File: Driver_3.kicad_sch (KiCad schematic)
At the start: 32 parts

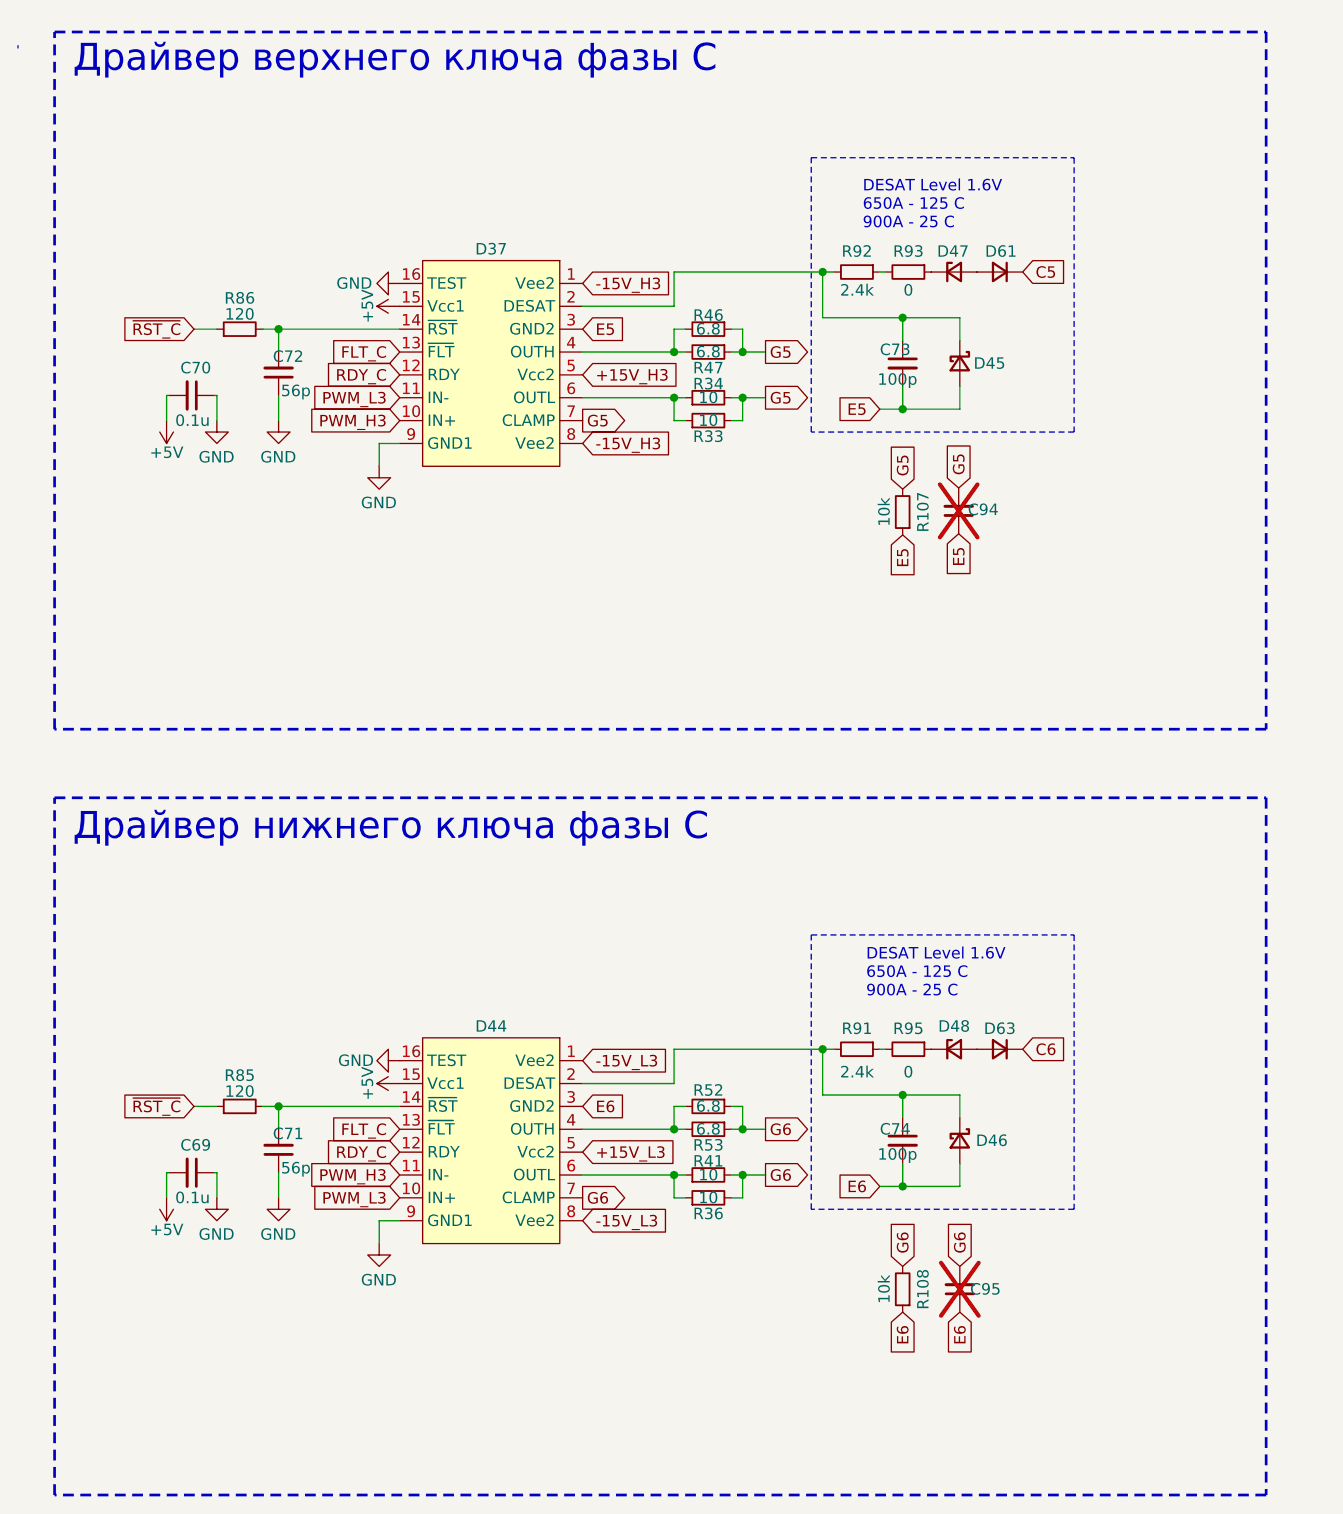
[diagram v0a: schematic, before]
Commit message: VER2.2.1: создал папку для производственных доков
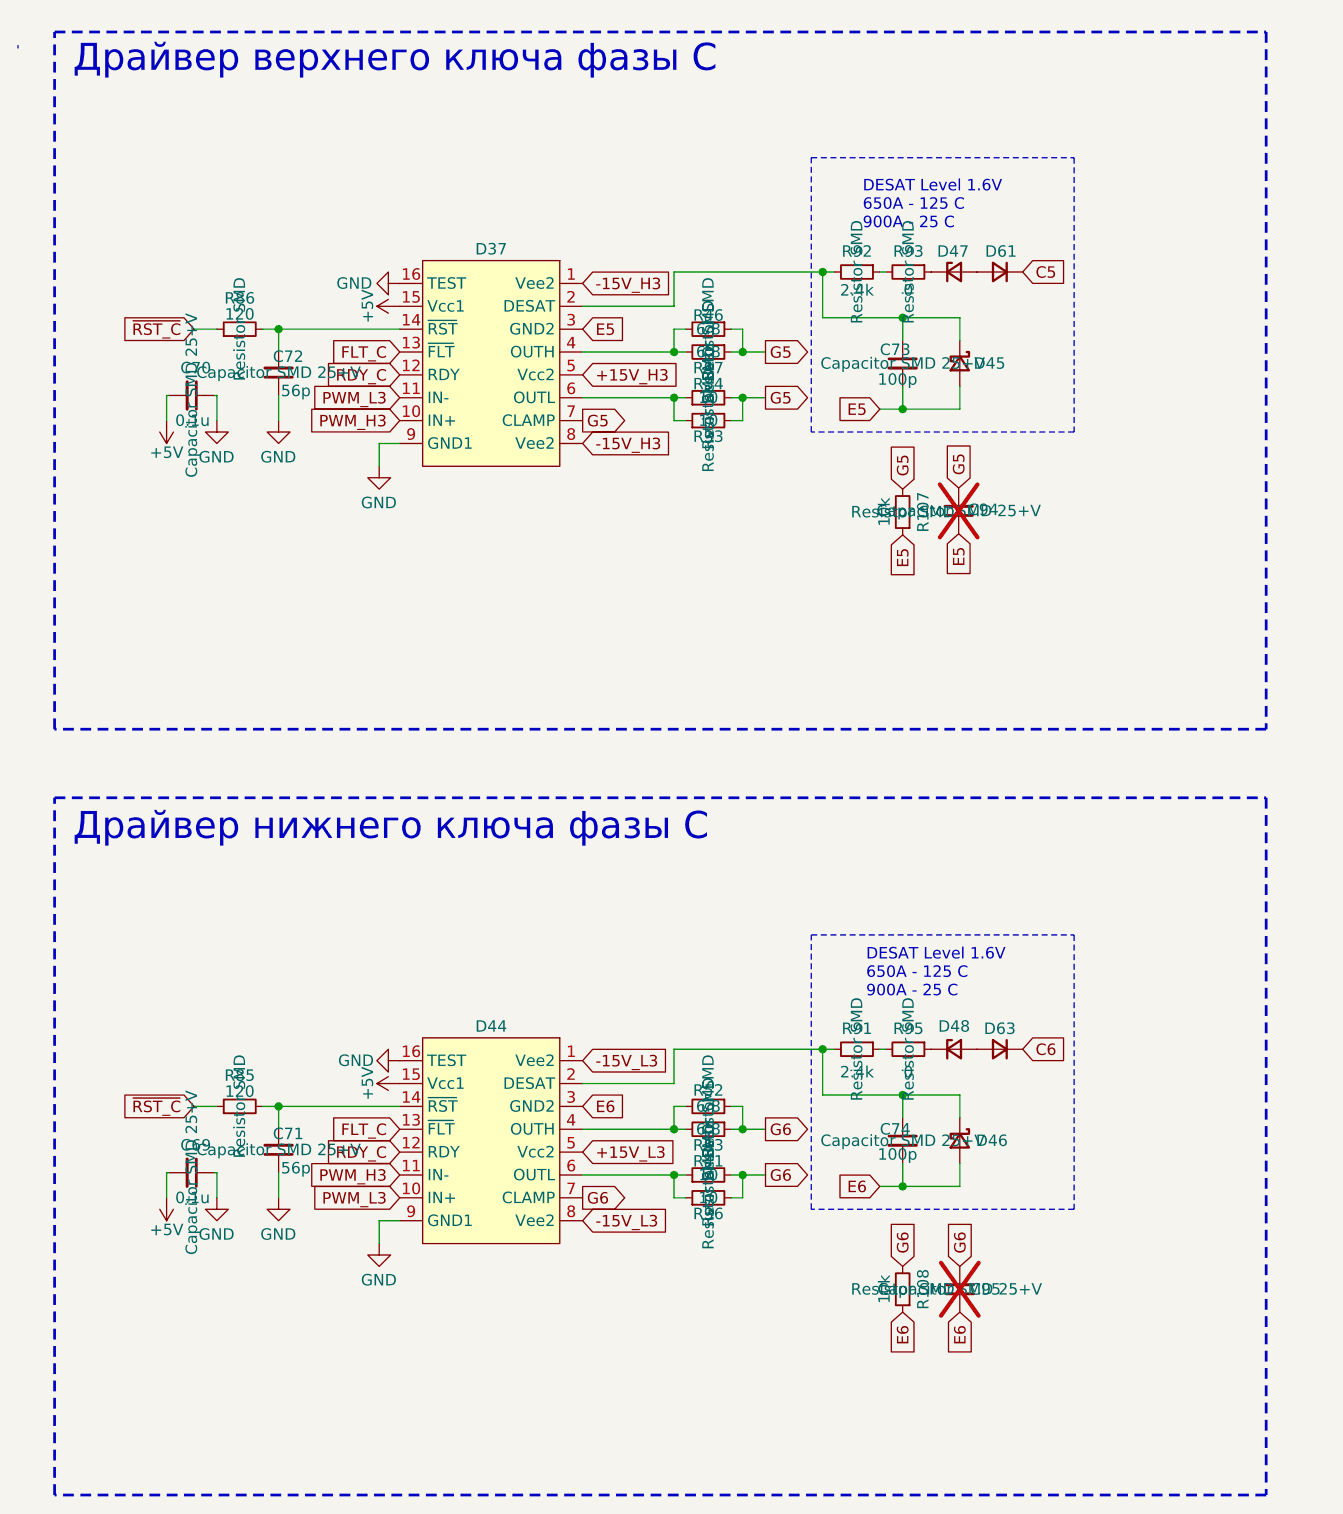
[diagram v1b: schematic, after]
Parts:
- C69, C70, C71, C72, C73, C74, C94, C95: Description P/N (none) -> Capacitor SMD 25+V
- R107, R108, R33, R34, R36, R41, R46, R47, R52, R53, R85, R86, R91, R92, R93, R95: Description P/N (none) -> Resistor SMD
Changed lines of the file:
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@@
 			)
 		)
-		(property "Description P/N" ""
+		(property "Description P/N" "Capacitor SMD 25+V"
 			(at 181.61 162.56 0)
 			(effects
@@
 			)
 		)
-		(property "Description P/N" ""
+		(property "Description P/N" "Resistor SMD"
 			(at 153.67 152.4 0)
 			(effects
@@
 			)
 		)
-		(property "Description P/N" ""
+		(property "Description P/N" "Capacitor SMD 25+V"
 			(at 105.918 60.706 0)
 			(effects
@@
 			)
 		)
-		(property "Description P/N" ""
+		(property "Description P/N" "Resistor SMD"
 			(at 153.67 149.86 0)
 			(effects
@@
 			)
 		)
-		(property "Description P/N" ""
+		(property "Description P/N" "Capacitor SMD 25+V"
 			(at 105.918 147.066 0)
 			(effects
@@
 			)
 		)
-		(property "Description P/N" ""
+		(property "Description P/N" "Resistor SMD"
 			(at 175.26 162.56 0)
 			(effects
@@
 			)
 		)
-		(property "Description P/N" ""
+		(property "Description P/N" "Capacitor SMD 25+V"
 			(at 175.26 59.69 0)
 			(effects
@@
 			)
 		)
-		(property "Description P/N" ""
+		(property "Description P/N" "Resistor SMD"
 			(at 153.67 66.04 0)
 			(effects
@@
 			)
 		)
-		(property "Description P/N" ""
+		(property "Description P/N" "Resistor SMD"
 			(at 170.18 135.89 0)
 			(effects
@@
 			)
 		)
-		(property "Description P/N" ""
+		(property "Description P/N" "Resistor SMD"
 			(at 175.26 76.2 0)
 			(effects
@@
 			)
 		)
-		(property "Description P/N" ""
+		(property "Description P/N" "Capacitor SMD 25+V"
 			(at 181.483 76.073 0)
 			(effects
@@
 			)
 		)
-		(property "Description P/N" ""
+		(property "Description P/N" "Resistor SMD"
 			(at 175.895 49.53 0)
 			(effects
@@
 			)
 		)
-		(property "Description P/N" ""
+		(property "Description P/N" "Resistor SMD"
 			(at 153.67 142.24 0)
 			(effects
@@
 			)
 		)
-		(property "Description P/N" ""
+		(property "Description P/N" "Resistor SMD"
 			(at 101.6 142.24 0)
 			(effects
@@
 			)
 		)
-		(property "Description P/N" ""
+		(property "Description P/N" "Capacitor SMD 25+V"
 			(at 175.26 146.05 0)
 			(effects
@@
 			)
 		)
-		(property "Description P/N" ""
+		(property "Description P/N" "Resistor SMD"
 			(at 153.67 58.42 0)
 			(effects
@@
 			)
 		)
-		(property "Description P/N" ""
+		(property "Description P/N" "Resistor SMD"
 			(at 153.67 63.5 0)
 			(effects
@@
 			)
 		)
-		(property "Description P/N" ""
+		(property "Description P/N" "Resistor SMD"
 			(at 153.67 144.78 0)
 			(effects
@@
 			)
 		)
-		(property "Description P/N" ""
+		(property "Description P/N" "Resistor SMD"
 			(at 170.18 49.53 0)
 			(effects
@@
 			)
 		)
-		(property "Description P/N" ""
+		(property "Description P/N" "Resistor SMD"
 			(at 101.6 55.88 0)
 			(effects
@@
 			)
 		)
-		(property "Description P/N" ""
+		(property "Description P/N" "Resistor SMD"
 			(at 175.895 135.89 0)
 			(effects
@@
 			)
 		)
-		(property "Description P/N" ""
+		(property "Description P/N" "Capacitor SMD 25+V"
 			(at 96.266 149.606 0)
 			(effects
@@
 			)
 		)
-		(property "Description P/N" ""
+		(property "Description P/N" "Capacitor SMD 25+V"
 			(at 96.266 63.246 0)
 			(effects
@@
 			)
 		)
-		(property "Description P/N" ""
+		(property "Description P/N" "Resistor SMD"
 			(at 153.67 55.88 0)
 			(effects

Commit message: VER2.2.1: исправил все доки
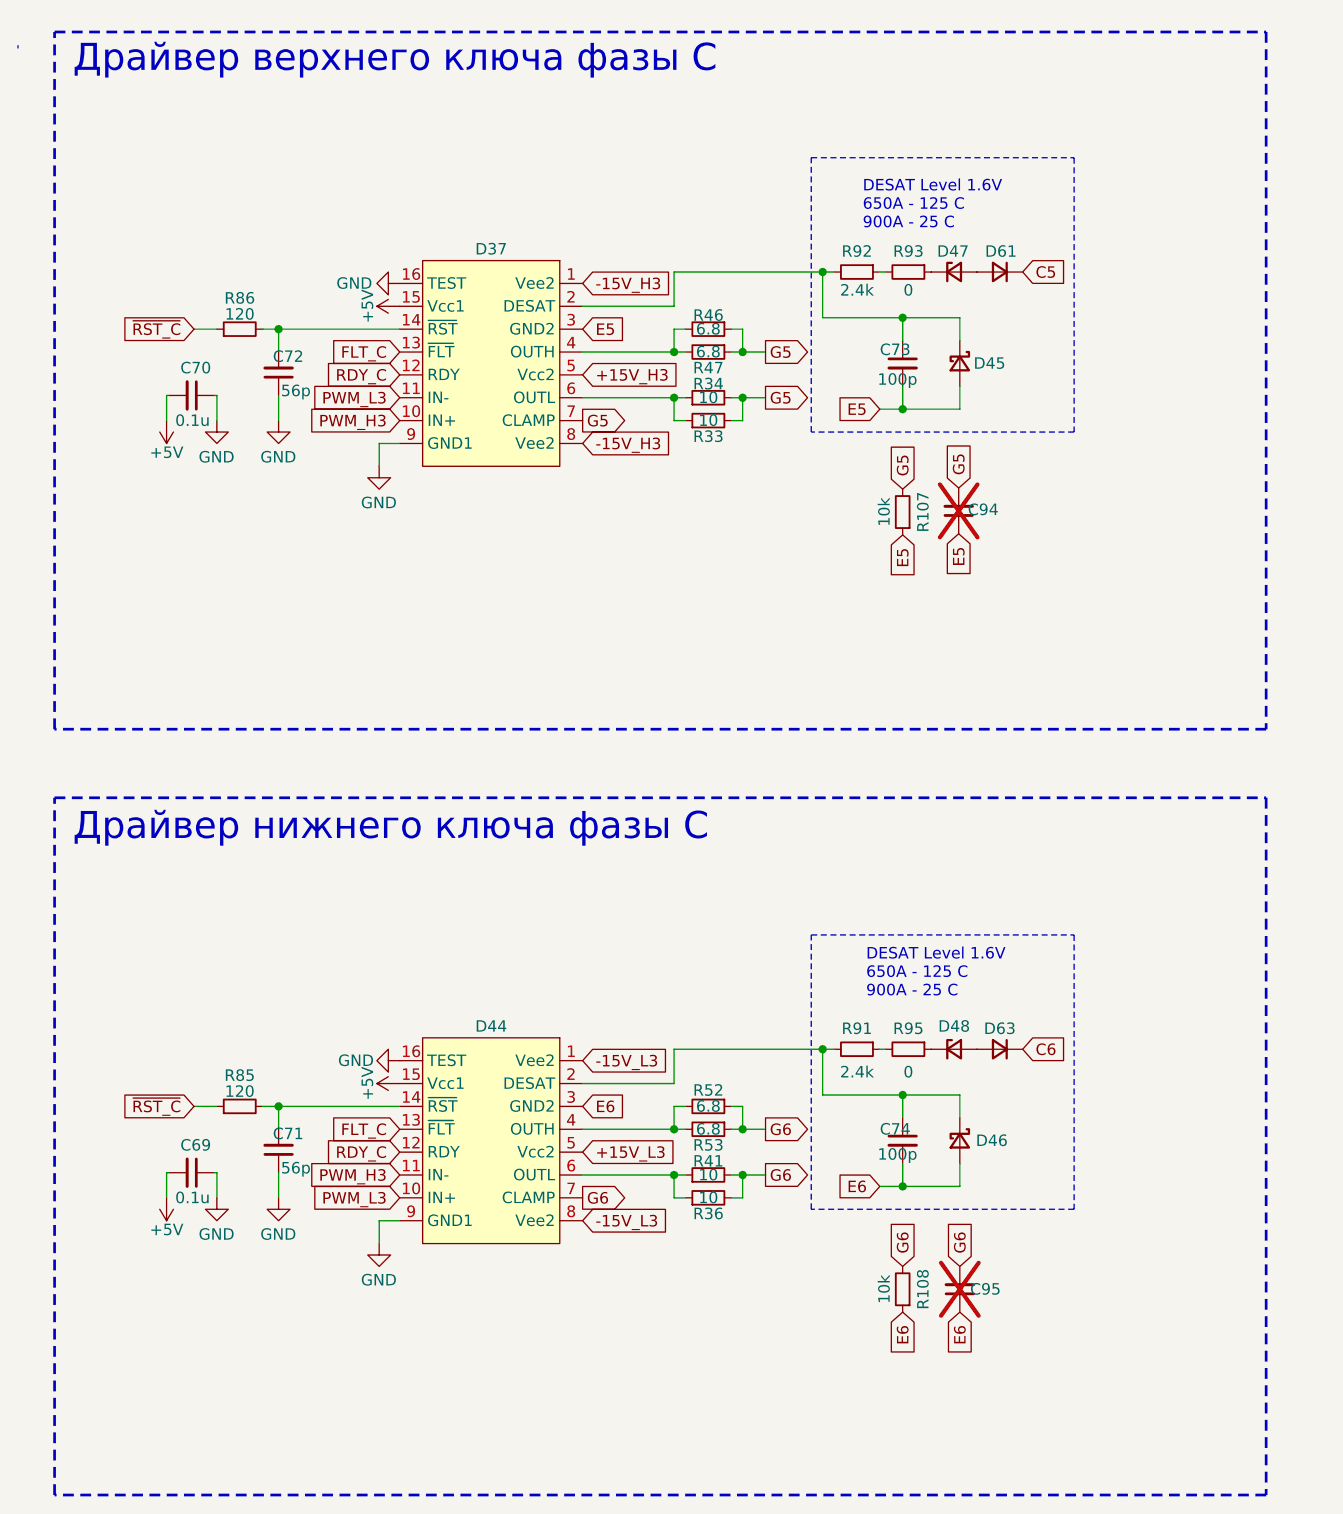
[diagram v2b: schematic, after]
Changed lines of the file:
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@@
 		(date "2025-06-04")
 		(company "ООО \"ЭТТ\"")
+		(comment 1 "НВЦТ.EVP150-2-1.2000.120_v1 Э3")
 	)
 	(rectangle
@@
 				)
 				(justify left)
+				(hide yes)
 			)
 		)
@@
 					(size 1.27 1.27)
 				)
+				(hide yes)
 			)
 		)
@@
 					(size 1.27 1.27)
 				)
+				(hide yes)
 			)
 		)
@@
 					(size 1.27 1.27)
 				)
+				(hide yes)
 			)
 		)
@@
 					(size 1.27 1.27)
 				)
+				(hide yes)
 			)
 		)
@@
 					(size 1.27 1.27)
 				)
+				(hide yes)
 			)
 		)
@@
 					(size 1.27 1.27)
 				)
+				(hide yes)
 			)
 		)
@@
 					(size 1.27 1.27)
 				)
+				(hide yes)
 			)
 		)
@@
 					(size 1.27 1.27)
 				)
+				(hide yes)
 			)
 		)
@@
 					(size 1.27 1.27)
 				)
+				(hide yes)
 			)
 		)
@@
 					(size 1.27 1.27)
 				)
+				(hide yes)
 			)
 		)
@@
 				)
 				(justify left)
+				(hide yes)
 			)
 		)
@@
 					(size 1.27 1.27)
 				)
+				(hide yes)
 			)
 		)
@@
 					(size 1.27 1.27)
 				)
+				(hide yes)
 			)
 		)
@@
 					(size 1.27 1.27)
 				)
+				(hide yes)
 			)
 		)
@@
 					(size 1.27 1.27)
 				)
+				(hide yes)
 			)
 		)
@@
 					(size 1.27 1.27)
 				)
+				(hide yes)
 			)
 		)
@@
 					(size 1.27 1.27)
 				)
+				(hide yes)
 			)
 		)
@@
 					(size 1.27 1.27)
 				)
+				(hide yes)
 			)
 		)
@@
 					(size 1.27 1.27)
 				)
+				(hide yes)
 			)
 		)
@@
 					(size 1.27 1.27)
 				)
+				(hide yes)
 			)
 		)
@@
 					(size 1.27 1.27)
 				)
+				(hide yes)
 			)
 		)
@@
 					(size 1.27 1.27)
 				)
+				(hide yes)
 			)
 		)
@@
 					(size 1.27 1.27)
 				)
+				(hide yes)
 			)
 		)
@@
 					(size 1.27 1.27)
 				)
+				(hide yes)
 			)
 		)
@@
 					(size 1.27 1.27)
 				)
+				(hide yes)
 			)
 		)

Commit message: VER2.2: исправил ошибки в доках
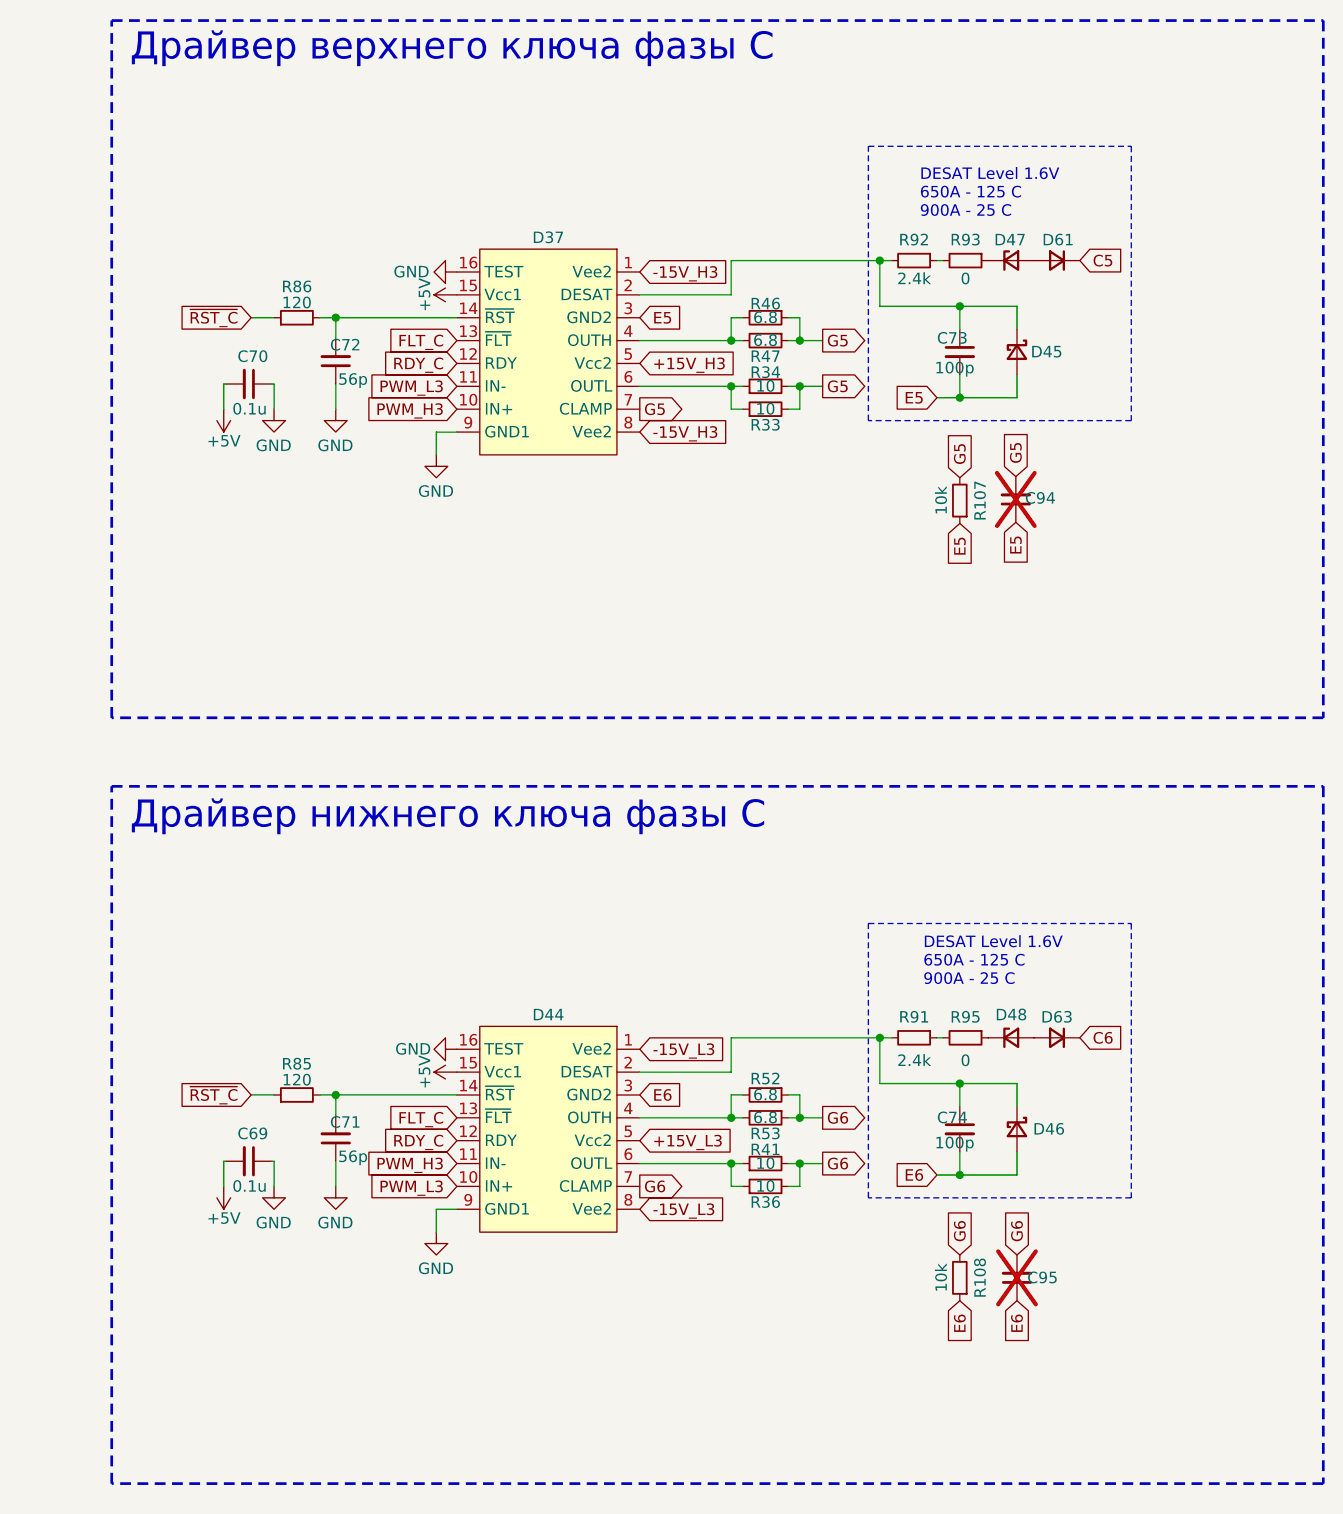
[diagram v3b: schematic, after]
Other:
- moved on the sheet: C69, C70, C71, C72, C73, C74, C94, C95, D37, D44, D45, D46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
